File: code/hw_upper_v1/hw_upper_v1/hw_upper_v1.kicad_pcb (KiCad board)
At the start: 2 copper layers, 102 x 49 mm, 11 parts, among them J1 Conn_02x20_Odd_Even

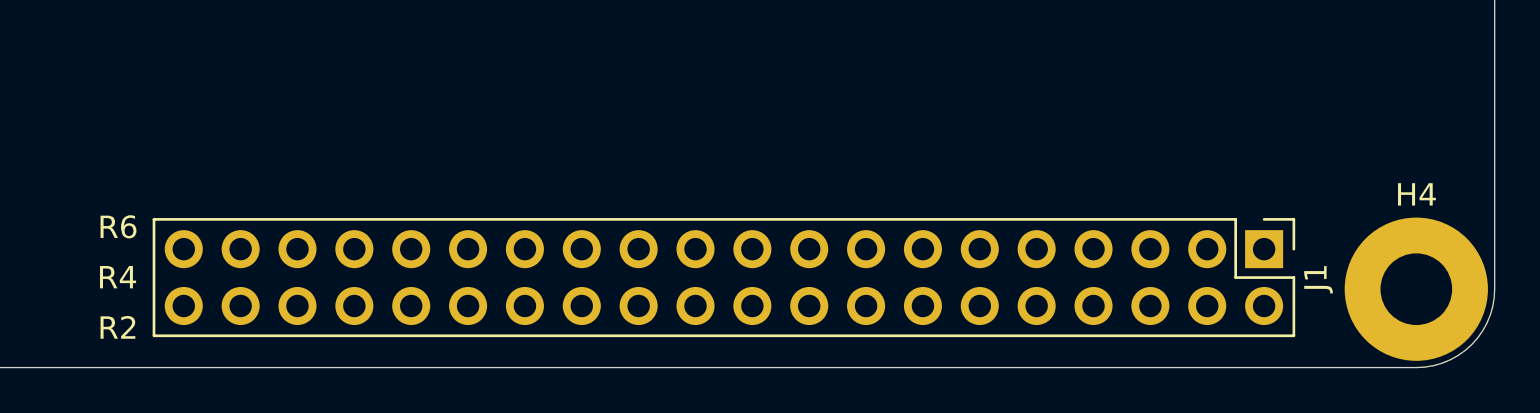
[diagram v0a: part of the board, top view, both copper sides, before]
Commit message: before the final route
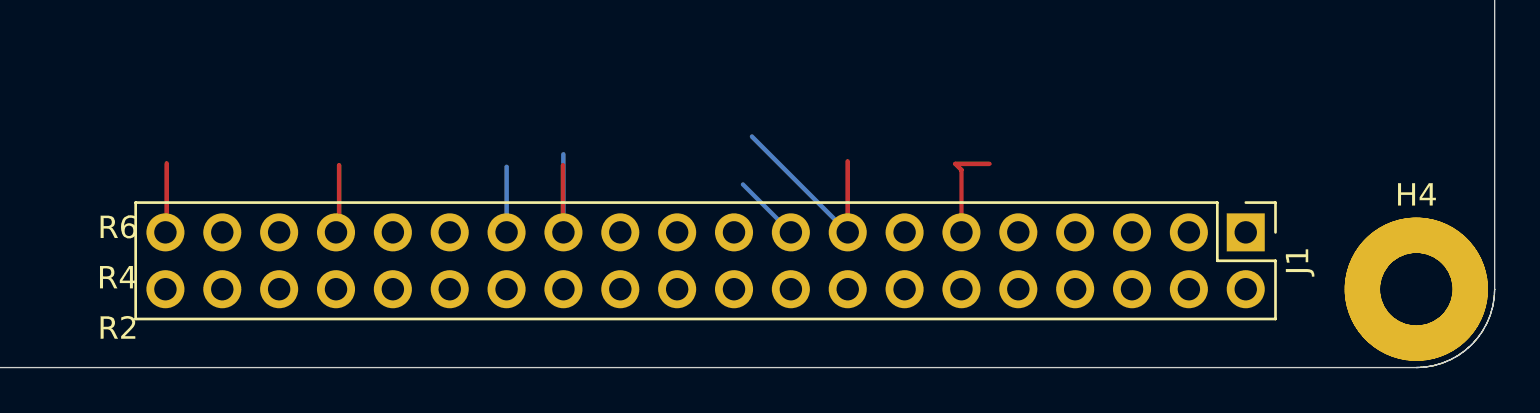
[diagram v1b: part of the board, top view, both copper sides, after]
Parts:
- added H5: MountingHole, MountingHole:MountingHole_3.2mm_M3_Pad, F.Cu at (192.5, 118.0)
- moved J1 1.11 mm to (184.9, 115.5)
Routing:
- net unconnected-(J1-Pin_15-Pad15): track 0.00 -> 9.23 mm
- net unconnected-(J1-Pin_25-Pad25): track 0.00 -> 6.50 mm
- net unconnected-(J1-Pin_11-Pad11): track 0.00 -> 4.69 mm
- net unconnected-(J1-Pin_39-Pad39): track 0.00 -> 3.11 mm
- net unconnected-(J1-Pin_33-Pad33): track 0.00 -> 3.06 mm
- net unconnected-(J1-Pin_17-Pad17): track 0.00 -> 3.03 mm
- net unconnected-(J1-Pin_27-Pad27): track 0.00 -> 2.93 mm
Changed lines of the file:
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@@
 	(footprint "Connector_PinHeader_2.54mm:PinHeader_2x20_P2.54mm_Vertical"
 		(layer "F.Cu")
-		(at 185.7 116.21 -90)
+		(at 184.88 115.46 -90)
 		(descr "Through hole straight pin header, 2x20, 2.54mm pitch, double rows")
 		(tags "Through hole pin header THT 2x20 2.54mm double row")
@@
 		)
 		(fp_text user "${REFERENCE}"
-			(at 1.27 24.13 360)
+			(at 1.27 24.13 0)
 			(layer "F.Fab")
 			(effects
@@
 	(footprint "MountingHole:MountingHole_3.2mm_M3_Pad"
 		(layer "F.Cu")
+		(at 192.5 118 -90)
+		(descr "Mounting Hole 3.2mm, M3")
+		(tags "mounting hole 3.2mm m3")
+		(property "Reference" "H5"
+			(at 0 -4.2 -90)
+			(layer "F.SilkS")
+			(hide yes)
+			(effects
+				(font
+					(size 1 1)
+					(thickness 0.15)
+				)
+			)
+		)
+		(property "Value" "MountingHole"
+			(at 0 4.2 -90)
+			(layer "F.Fab")
+			(effects
+				(font
+					(size 1 1)
+					(thickness 0.15)
+				)
+			)
+		)
+		(property "Footprint" "MountingHole:MountingHole_3.2mm_M3_Pad"
+			(at 0 0 -90)
+			(unlocked yes)
+			(layer "F.Fab")
+			(hide yes)
+			(effects
+				(font
+					(size 1.27 1.27)
+					(thickness 0.15)
+				)
+			)
+		)
+		(property "Datasheet" ""
+			(at 0 0 -90)
+			(unlocked yes)
+			(layer "F.Fab")
+			(hide yes)
+			(effects
+				(font
+					(size 1.27 1.27)
+					(thickness 0.15)
+				)
+			)
+		)
+		(property "Description" "Mounting Hole without connection"
+			(at 0 0 -90)
+			(unlocked yes)
+			(layer "F.Fab")
+			(hide yes)
+			(effects
+				(font
+					(size 1.27 1.27)
+					(thickness 0.15)
+				)
+			)
+		)
+		(property "Name" ""
+			(at 0 0 -90)
+			(unlocked yes)
+			(layer "F.Fab")
+			(hide yes)
+			(effects
+				(font
+					(size 1 1)
+					(thickness 0.15)
+				)
+			)
+		)
+		(attr exclude_from_pos_files exclude_from_bom)
+		(fp_circle
+			(center 0 0)
+			(end 3.2 0)
+			(stroke
+				(width 0.15)
+				(type solid)
+			)
+			(fill none)
+			(layer "Cmts.User")
+		)
+		(fp_circle
+			(center 0 0)
+			(end 3.45 0)
+			(stroke
+				(width 0.05)
+				(type solid)
+			)
+			(fill none)
+			(layer "F.CrtYd")
+		)
+		(fp_text user "${REFERENCE}"
+			(at 0 0 -90)
+			(layer "F.Fab")
+			(effects
+				(font
+					(size 1 1)
+					(thickness 0.15)
+				)
+			)
+		)
+		(pad "1" thru_hole circle
+			(at 0 0 270)
+			(size 6.4 6.4)
+			(drill 3.2)
+			(layers "*.Cu" "*.Mask")
+			(remove_unused_layers no)
+		)
+	)
+	(footprint "MountingHole:MountingHole_3.2mm_M3_Pad"
+		(layer "F.Cu")
 		(at 97.5 76)
 		(descr "Mounting Hole 3.2mm, M3")
@@
 		(layer "Edge.Cuts")
 	)
+	(gr_arc
+		(start 196 118)
+		(mid 194.974874 120.474874)
+		(end 192.5 121.5)
+		(stroke
+			(width 0.05)
+			(type default)
+		)
+		(layer "Edge.Cuts")
+	)
 	(gr_line
 		(start 192.5 121.5)
@@
 		)
 	)
+	(segment
+		(start 173.43 112.4)
+		(end 171.91 112.4)
+		(width 0.2)
+		(layer "F.Cu")
+		(net 1)
+	)
+	(segment
+		(start 172.18 112.67)
+		(end 172.18 115.46)
+		(width 0.2)
+		(layer "F.Cu")
+		(net 1)
+	)
+	(segment
+		(start 171.91 112.4)
+		(end 172.18 112.67)
+		(width 0.2)
+		(layer "F.Cu")
+		(net 1)
+	)
+	(segment
+		(start 144.38 115.32)
+		(end 144.24 115.46)
+		(width 0.2)
+		(layer "F.Cu")
+		(net 7)
+	)
+	(segment
+		(start 144.38 112.46)
+		(end 144.38 115.32)
+		(width 0.2)
+		(layer "F.Cu")
+		(net 7)
+	)
+	(segment
+		(start 139.13 118)
+		(end 139.16 118)
+		(width 0.2)
+		(layer "B.Cu")
+		(net 10)
+	)
+	(segment
+		(start 164.56 115.46)
+		(end 162.42 113.32)
+		(width 0.2)
+		(layer "B.Cu")
+		(net 11)
+	)
+	(segment
+		(start 136.68 115.4)
+		(end 136.62 115.46)
+		(width 0.2)
+		(layer "F.Cu")
+		(net 15)
+	)
+	(segment
+		(start 136.68 112.375)
+		(end 136.68 115.4)
+		(width 0.2)
+		(layer "F.Cu")
+		(net 15)
+	)
+	(segment
+		(start 151.86 112.53)
+		(end 151.86 115.46)
+		(width 0.2)
+		(layer "B.Cu")
+		(net 17)
+	)
+	(segment
+		(start 167.1 112.285)
+		(end 167.1 115.46)
+		(width 0.2)
+		(layer "F.Cu")
+		(net 27)
+	)
+	(segment
+		(start 162.82 111.18)
+		(end 167.1 115.46)
+		(width 0.2)
+		(layer "B.Cu")
+		(net 27)
+	)
+	(segment
+		(start 154.38 112.46)
+		(end 154.38 115.44)
+		(width 0.2)
+		(layer "F.Cu")
+		(net 30)
+	)
+	(segment
+		(start 154.38 115.44)
+		(end 154.4 115.46)
+		(width 0.2)
+		(layer "F.Cu")
+		(net 30)
+	)
+	(segment
+		(start 154.4 111.97)
+		(end 154.4 115.46)
+		(width 0.2)
+		(layer "B.Cu")
+		(net 30)
+	)
+	(segment
+		(start 161.88 115.32)
+		(end 162.02 115.46)
+		(width 0.2)
+		(layer "F.Cu")
+		(net 38)
+	)
 	(group ""
